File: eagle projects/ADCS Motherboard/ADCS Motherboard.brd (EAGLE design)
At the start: 91 x 91 mm, 142 parts, among them J1 HDR_10_EZFET_DEBUGGER, J11 CNC_3221-10-0300-00, J3 CNC_3221-10-0300-00, J5 CNC_3221-10-0300-00, J7 TE-1734829-3, Q1 PMV16XN, Q2 IRLML6246TRPBF, Q3 IRLML2246TRPBF, U1 MSP430F5529IPN, U10 TSV991AILT, U2 TSV991AILT, U3 ADS7841E_2K5, U4 TSV991AILT, U7 HMC1053, U9 BMX160, Y1 32.768kHz, Y2 CSTCR4M00G15L99, Y3 32.768kHz

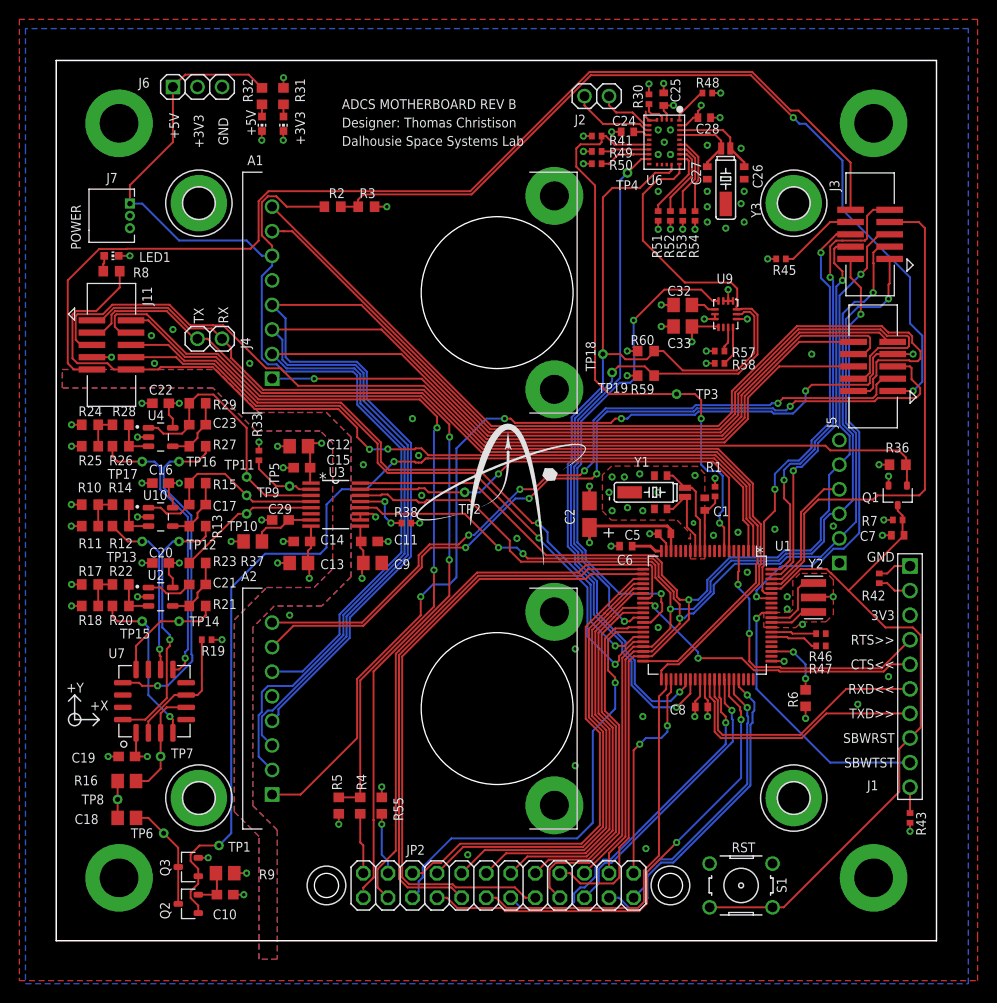
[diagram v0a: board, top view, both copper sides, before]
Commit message: Rev B almost ready
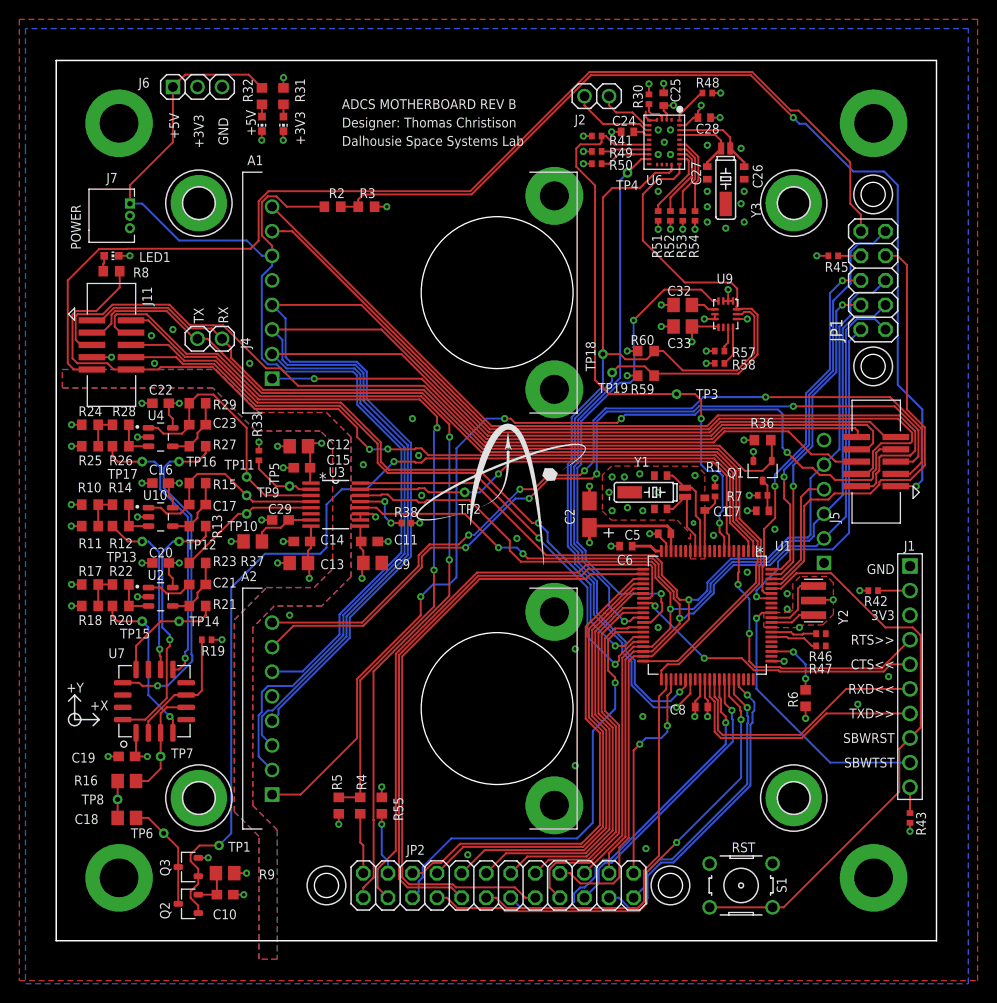
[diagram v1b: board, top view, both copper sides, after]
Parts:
- removed J3: CNC_3221-10-0300-00, my_library:CNC_3221-10-0300-00
- added JP1: (no value), pinhead:2X05
- moved C7 14.2 mm to (73.0, 44.5)
- moved Q1 14.2 mm to (73.0, 48.6)
- moved R36 14.2 mm to (73.0, 51.8)
- moved R7 14.2 mm to (73.0, 46.0)
- moved J5 9.85 mm to (84.8, 49.5)
- moved R45 5.41 mm to (80.3, 70.8)
- moved JP4 1.59 mm to (79.4, 45.4)
- moved R42 1.42 mm to (84.5, 36.2), turned to 180 degrees
- moved Y2 0.32 mm to (78.3, 35.2)
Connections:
- net !CS!_SUN_X+: now also JP1.2; no longer J3.2
- net !CS!_SUN_X-: now also JP1.7; no longer J3.7
- net !CS!_SUN_Y+: now also JP1.4; no longer J3.4
- net !CS!_SUN_Y-: now also JP1.9; no longer J3.9
- net !CS!_SUN_Z-: now also JP1.6; no longer J3.6
- net N$58: now also JP1.8; no longer J3.8
- net UCB0_SPI_CLK: now also JP1.5; no longer J3.5
- net UCB0_SPI_MISO: now also JP1.1; no longer J3.1
- net UCB0_SPI_MOSI: now also JP1.3; no longer J3.3
- net Z-_SUN_3V_PRESENT: now also JP1.10; no longer J3.10
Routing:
- net MSP_OBC_RESET: track 100.2 -> 86.6 mm
- net CAM_5V_PRESENT: track 93.1 -> 104.7 mm
- net CAMERA-2_SCL: track 78.4 -> 87.9 mm
- net UCB0_SPI_MOSI: track 127.0 -> 118.2 mm, vias 2 -> 1
- net !CS!_SUN_X+: track 45.1 -> 36.3 mm, vias 2 -> 1
- net RST/SBWTDIO: track 72.2 -> 63.8 mm
- net UCB0_SPI_MISO: track 124.4 -> 116.6 mm, vias 4 -> 3
- net UCB0_SPI_CLK: track 132.7 -> 126.1 mm, vias 2 -> 1
- net !CS!_SUN_Y+: track 39.7 -> 33.3 mm
- net N$58: track 8.27 -> 2.36 mm
- net CAMERA-1_SCL: track 94.0 -> 88.1 mm
- net !CS!_SUN_Z-: track 43.9 -> 38.5 mm
- net !CS!_SUN_X-: track 53.7 -> 48.5 mm
- net !CS!_SUN_Y-: track 46.9 -> 41.8 mm, vias 2 -> 1
- net CAMERA_SCLK: track 134.5 -> 130.0 mm
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
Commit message: Idk what i changed
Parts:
- Q1: value PMV16XN -> BSR802NL6327HTSA1
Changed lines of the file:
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@@
 <attribute name="SPICEPREFIX" value="R" x="73.025" y="51.7525" size="1.778" layer="27" display="off"/>
 </element>
-<element name="Q1" library="my_library" library_urn="urn:adsk.eagle:library:22876504" package="SOT23-3P95_230X110L20X43N_PMV16XN" package3d_urn="urn:adsk.eagle:package:24628515/1" value="PMV16XN" x="73.025" y="48.5775" smashed="yes" rot="R180">
+<element name="Q1" library="my_library" library_urn="urn:adsk.eagle:library:22876504" package="SOT23-3P95_230X110L20X43N_PMV16XN" package3d_urn="urn:adsk.eagle:package:24628515/1" value="BSR802NL6327HTSA1" x="73.025" y="48.5775" smashed="yes" rot="R180">
 <attribute name="NAME" x="71.12" y="48.895" size="1.016" layer="25" ratio="10" rot="R180"/>
 </element>
